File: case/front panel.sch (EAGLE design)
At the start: 3 parts, among them J16 8pin

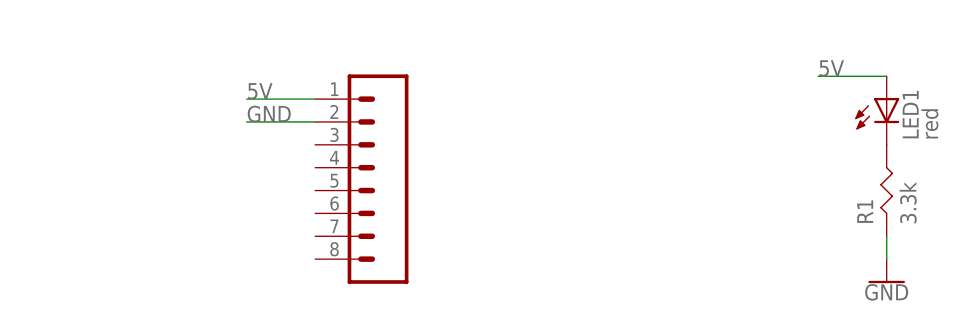
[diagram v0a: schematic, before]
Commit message: front panel pcb v1.0
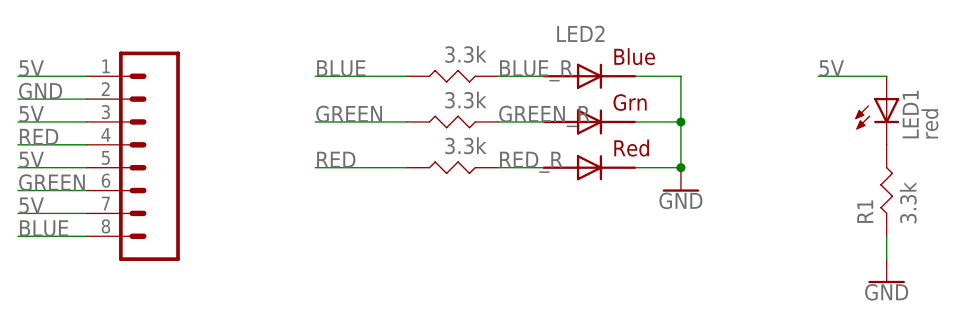
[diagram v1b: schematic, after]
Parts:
- added LED2: RGBLED5050, adafruit:RGBLED5050
- added R2, R3, R4: 3.3k, FlashPCB_Resistors:RES-0402
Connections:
- new net BLUE: J16.8, R2.P$2
- new net BLUE_R: LED2.BLUE_A, R2.P$1
- new net GREEN: J16.6, R3.P$2
- new net GREEN_R: LED2.GREEN_A, R3.P$1
- new net RED: J16.4, R4.P$2
- new net RED_R: LED2.RED_A, R4.P$1
- net 5V: now also J16.3, J16.5, J16.7
- net GND: now also LED2.BLUE_C, LED2.GREEN_C, LED2.RED_C
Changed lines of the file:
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@@
 <part name="R1" library="FlashPCB_Resistors" deviceset="RES-0402" device="" value="3.3k"/>
 <part name="LED1" library="adafruit" library_urn="urn:adsk.eagle:library:420" deviceset="LED" device="CHIP-LED0603" package3d_urn="urn:adsk.eagle:package:6240556/1" value="red"/>
+<part name="LED2" library="adafruit" library_urn="urn:adsk.eagle:library:420" deviceset="RGBLED" device="5050" package3d_urn="urn:adsk.eagle:package:6240865/1"/>
+<part name="GND1" library="SparkFun-PowerSymbols" library_urn="urn:adsk.eagle:library:530" deviceset="GND" device=""/>
+<part name="R2" library="FlashPCB_Resistors" deviceset="RES-0402" device="" value="3.3k"/>
+<part name="R3" library="FlashPCB_Resistors" deviceset="RES-0402" device="" value="3.3k"/>
+<part name="R4" library="FlashPCB_Resistors" deviceset="RES-0402" device="" value="3.3k"/>
 </parts>
 <sheets>
@@
 </plain>
 <instances>
-<instance part="J16" gate="G$1" x="35.56" y="20.32" smashed="yes" rot="R180"/>
+<instance part="J16" gate="G$1" x="10.16" y="22.86" smashed="yes" rot="R180"/>
 <instance part="GND2" gate="1" x="93.98" y="7.62" smashed="yes">
 <attribute name="VALUE" x="93.98" y="7.366" size="1.778" layer="96" align="top-center"/>
@@
 <attribute name="NAME" x="97.536" y="23.368" size="1.778" layer="95" rot="R90"/>
 <attribute name="VALUE" x="99.695" y="23.368" size="1.778" layer="96" rot="R90"/>
+</instance>
+<instance part="LED2" gate="G$1" x="60.96" y="25.4" smashed="yes">
+<attribute name="NAME" x="57.15" y="34.29" size="1.778" layer="95"/>
+</instance>
+<instance part="GND1" gate="1" x="71.12" y="17.78" smashed="yes">
+<attribute name="VALUE" x="71.12" y="17.526" size="1.778" layer="96" align="top-center"/>
+</instance>
+<instance part="R2" gate="G$1" x="45.72" y="30.48" smashed="yes" rot="R180">
+<attribute name="VALUE" x="49.53" y="33.782" size="1.778" layer="96" rot="R180"/>
+</instance>
+<instance part="R3" gate="G$1" x="45.72" y="25.4" smashed="yes" rot="R180">
+<attribute name="VALUE" x="49.53" y="28.702" size="1.778" layer="96" rot="R180"/>
+</instance>
+<instance part="R4" gate="G$1" x="45.72" y="20.32" smashed="yes" rot="R180">
+<attribute name="VALUE" x="49.53" y="23.622" size="1.778" layer="96" rot="R180"/>
 </instance>
 </instances>
@@
 <segment>
 <pinref part="J16" gate="G$1" pin="2"/>
-<wire x1="30.48" y1="25.4" x2="22.86" y2="25.4" width="0.1524" layer="91"/>
-<label x="22.86" y="25.4" size="1.778" layer="95"/>
+<wire x1="5.08" y1="27.94" x2="-2.54" y2="27.94" width="0.1524" layer="91"/>
+<label x="-2.54" y="27.94" size="1.778" layer="95"/>
+</segment>
+<segment>
+<pinref part="LED2" gate="G$1" pin="RED_C"/>
+<wire x1="66.04" y1="20.32" x2="71.12" y2="20.32" width="0.1524" layer="91"/>
+<pinref part="GND1" gate="1" pin="GND"/>
+<pinref part="LED2" gate="G$1" pin="BLUE_C"/>
+<wire x1="66.04" y1="30.48" x2="71.12" y2="30.48" width="0.1524" layer="91"/>
+<pinref part="LED2" gate="G$1" pin="GREEN_C"/>
+<wire x1="66.04" y1="25.4" x2="71.12" y2="25.4" width="0.1524" layer="91"/>
+<wire x1="71.12" y1="30.48" x2="71.12" y2="25.4" width="0.1524" layer="91"/>
+<wire x1="71.12" y1="25.4" x2="71.12" y2="20.32" width="0.1524" layer="91"/>
+<junction x="71.12" y="25.4"/>
+<junction x="71.12" y="20.32"/>
 </segment>
 </net>
@@
 <segment>
 <pinref part="J16" gate="G$1" pin="1"/>
-<wire x1="30.48" y1="27.94" x2="22.86" y2="27.94" width="0.1524" layer="91"/>
-<label x="22.86" y="27.94" size="1.778" layer="95"/>
+<wire x1="5.08" y1="30.48" x2="-2.54" y2="30.48" width="0.1524" layer="91"/>
+<label x="-2.54" y="30.48" size="1.778" layer="95"/>
+</segment>
+<segment>
+<pinref part="J16" gate="G$1" pin="3"/>
+<wire x1="5.08" y1="25.4" x2="-2.54" y2="25.4" width="0.1524" layer="91"/>
+<label x="-2.54" y="25.4" size="1.778" layer="95"/>
+</segment>
+<segment>
+<pinref part="J16" gate="G$1" pin="5"/>
+<wire x1="5.08" y1="20.32" x2="-2.54" y2="20.32" width="0.1524" layer="91"/>
+<label x="-2.54" y="20.32" size="1.778" layer="95"/>
+</segment>
+<segment>
+<pinref part="J16" gate="G$1" pin="7"/>
+<wire x1="5.08" y1="15.24" x2="-2.54" y2="15.24" width="0.1524" layer="91"/>
+<label x="-2.54" y="15.24" size="1.778" layer="95"/>
 </segment>
 </net>
@@
 </segment>
 </net>
+<net name="BLUE" class="0">
+<segment>
+<pinref part="J16" gate="G$1" pin="8"/>
+<wire x1="5.08" y1="12.7" x2="-2.54" y2="12.7" width="0.1524" layer="91"/>
+<label x="-2.54" y="12.7" size="1.778" layer="95"/>
+</segment>
+<segment>
+<pinref part="R2" gate="G$1" pin="P$2"/>
+<wire x1="40.64" y1="30.48" x2="30.48" y2="30.48" width="0.1524" layer="91"/>
+<label x="30.48" y="30.48" size="1.778" layer="95"/>
+</segment>
+</net>
+<net name="GREEN" class="0">
+<segment>
+<pinref part="J16" gate="G$1" pin="6"/>
+<wire x1="5.08" y1="17.78" x2="-2.54" y2="17.78" width="0.1524" layer="91"/>
+<label x="-2.54" y="17.78" size="1.778" layer="95"/>
+</segment>
+<segment>
+<pinref part="R3" gate="G$1" pin="P$2"/>
+<wire x1="30.48" y1="25.4" x2="40.64" y2="25.4" width="0.1524" layer="91"/>
+<label x="30.48" y="25.4" size="1.778" layer="95"/>
+</segment>
+</net>
+<net name="RED" class="0">
+<segment>
+<pinref part="J16" gate="G$1" pin="4"/>
+<wire x1="5.08" y1="22.86" x2="-2.54" y2="22.86" width="0.1524" layer="91"/>
+<label x="-2.54" y="22.86" size="1.778" layer="95"/>
+</segment>
+<segment>
+<pinref part="R4" gate="G$1" pin="P$2"/>
+<wire x1="40.64" y1="20.32" x2="30.48" y2="20.32" width="0.1524" layer="91"/>
+<label x="30.48" y="20.32" size="1.778" layer="95"/>
+</segment>
+</net>
+<net name="BLUE_R" class="0">
+<segment>
+<pinref part="LED2" gate="G$1" pin="BLUE_A"/>
+<wire x1="55.88" y1="30.48" x2="50.8" y2="30.48" width="0.1524" layer="91"/>
+<label x="50.8" y="30.48" size="1.778" layer="95"/>
+<pinref part="R2" gate="G$1" pin="P$1"/>
+</segment>
+</net>
+<net name="GREEN_R" class="0">
+<segment>
+<pinref part="LED2" gate="G$1" pin="GREEN_A"/>
+<wire x1="55.88" y1="25.4" x2="50.8" y2="25.4" width="0.1524" layer="91"/>
+<label x="50.8" y="25.4" size="1.778" layer="95"/>
+<pinref part="R3" gate="G$1" pin="P$1"/>
+</segment>
+</net>
+<net name="RED_R" class="0">
+<segment>
+<pinref part="LED2" gate="G$1" pin="RED_A"/>
+<wire x1="55.88" y1="20.32" x2="50.8" y2="20.32" width="0.1524" layer="91"/>
+<label x="50.8" y="20.32" size="1.778" layer="95"/>
+<pinref part="R4" gate="G$1" pin="P$1"/>
+</segment>
+</net>
